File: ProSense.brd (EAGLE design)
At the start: 25.5 x 36.7 mm, 24 parts, among them U4 MIC2505 3.3

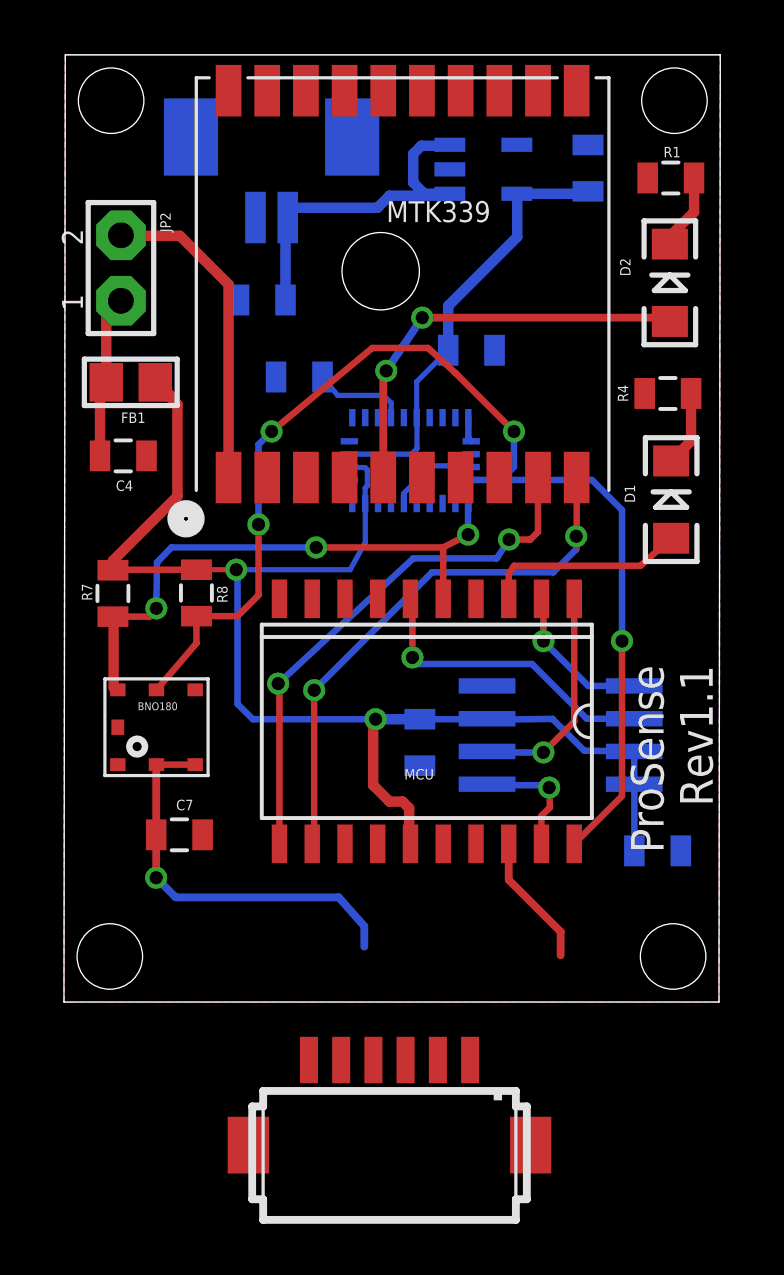
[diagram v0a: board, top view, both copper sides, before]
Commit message: Finished rev 1.2.1
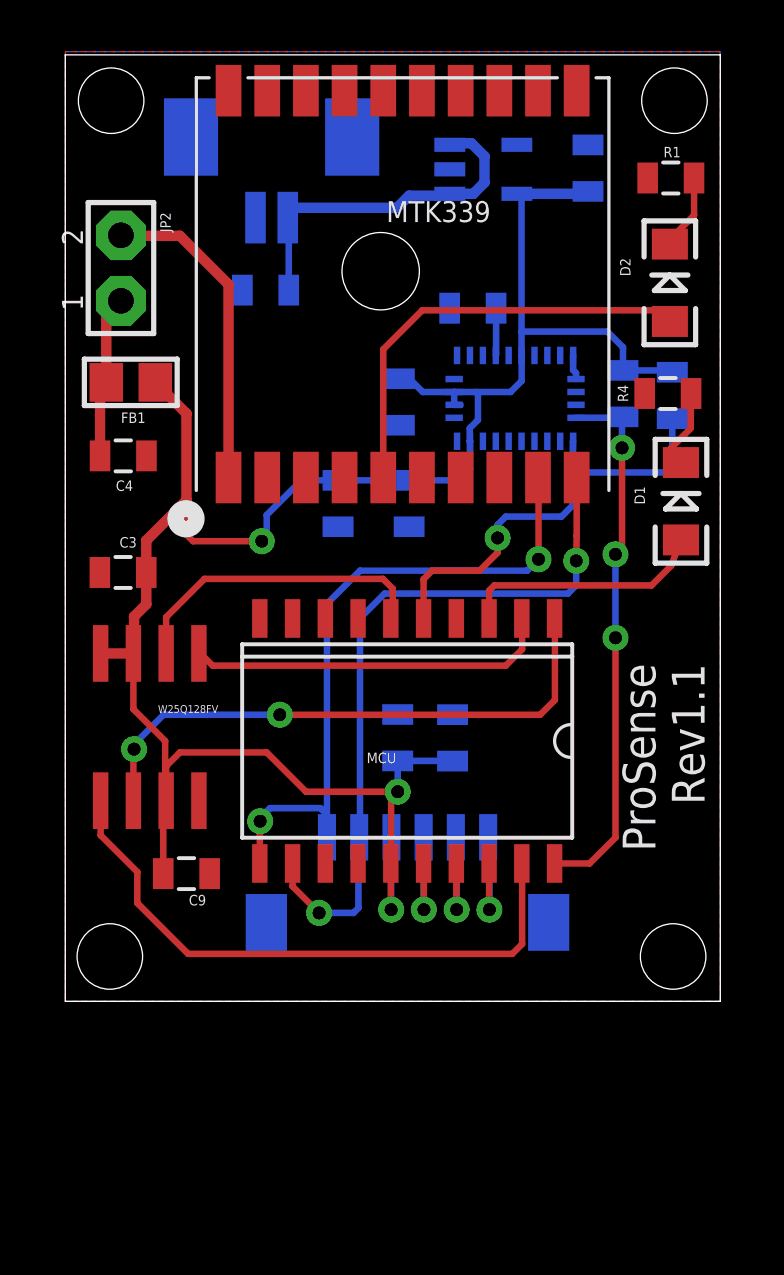
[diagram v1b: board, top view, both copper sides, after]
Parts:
- removed BNO180: BMP180, SparkFun-Sensors:BMP180
- added C1: 6.8nF, SparkFun-Passives:0805
- added C6, C9: .1uF, SparkFun-Passives:0805
- C2: value 10uF -> .1uF
- C5: value 4.7uF -> 120nF
- moved C3 23.4 mm to (37.8, 45.8), flipped to the top
- moved R7 21.2 mm to (57.2, 52.8), flipped to the bottom
- moved R8 20.0 mm to (59.1, 52.7), flipped to the bottom, turned to 90 degrees
- moved W25Q128FV 15.9 mm to (38.8, 39.8), flipped to the top, turned to 90 degrees
- moved C7 9.26 mm to (48.5, 39.4), flipped to the bottom, turned to 90 degrees
- moved U$1 8.66 mm to (48.8, 34.7), flipped to the bottom
- moved C5 7.88 mm to (46.1, 48.5), turned to 90 degrees
- moved C2 7.24 mm to (51.4, 56.1)
- moved BNO055 4.73 mm to (53.0, 52.6)
- moved C8 1.28 mm to (50.6, 39.4), turned to 90 degrees
- moved MCU 1.08 mm to (48.8, 39.3)
- moved C14 0.40 mm to (43.3, 56.8)
- moved D1 0.39 mm to (59.4, 48.6)
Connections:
- net N$6 renamed GPS-LED
- net GND: now also C1.1, C6.2, C9.1, U$1.P$4; no longer BNO180.7, U$1.P$3
- net ISP: now also U$1.P$6; no longer U$1.P$1
- net LPC_RX: now also U$1.P$1; no longer U$1.P$6
- net LPC_TX: now also U$1.P$2; no longer U$1.P$5
- net RESET: now also U$1.P$5; no longer U$1.P$2
- net SCL: now also R7.2; no longer BNO180.5, R8.2
- net SDA: now also R8.1; no longer BNO180.6, R7.2
- net VCC: now also C1.2, C6.1, C9.2, R8.2, U$1.P$3; no longer BNO180.2, BNO180.3, R8.1, U$1.P$4
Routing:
- net SCL: track 46.7 -> 21.1 mm, vias 4 -> 3
- net WS_CS: track 4.77 -> 23.6 mm, vias 1 -> 0
- net WS_DO: track 8.64 -> 22.4 mm, vias 1 -> 2
- net WS_DI: track 5.91 -> 14.2 mm, vias 1 -> 0
- net LPC_TX: track 21.9 -> 28.3 mm
- net LPC_RX: track 20.8 -> 25.8 mm
- net SDA: track 22.2 -> 17.4 mm, vias 3 -> 1
- net RESET: track 0.00 -> 4.61 mm, vias 0 -> 1
- net VCC: track 88.4 -> 84.5 mm
- net N$2: track 3.70 -> 1.84 mm
- net LPC_LED: track 7.84 -> 9.61 mm
- net GND: track 4.43 -> 5.57 mm, vias 0 -> 1
- net V_BATT: track 14.4 -> 13.9 mm
- net ISP: track 5.16 -> 4.62 mm, vias 0 -> 1
- net WS_SCK: track 11.9 -> 12.2 mm, vias 1 -> 0
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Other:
- board size 25.5 x 36.7 mm -> 25.4 x 36.7 mm
